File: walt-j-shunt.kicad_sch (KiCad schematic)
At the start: 32 parts, among them Q1 NMOS, Q2 NJVMJD45H11T4G, Q3 PNP, U1 AD817

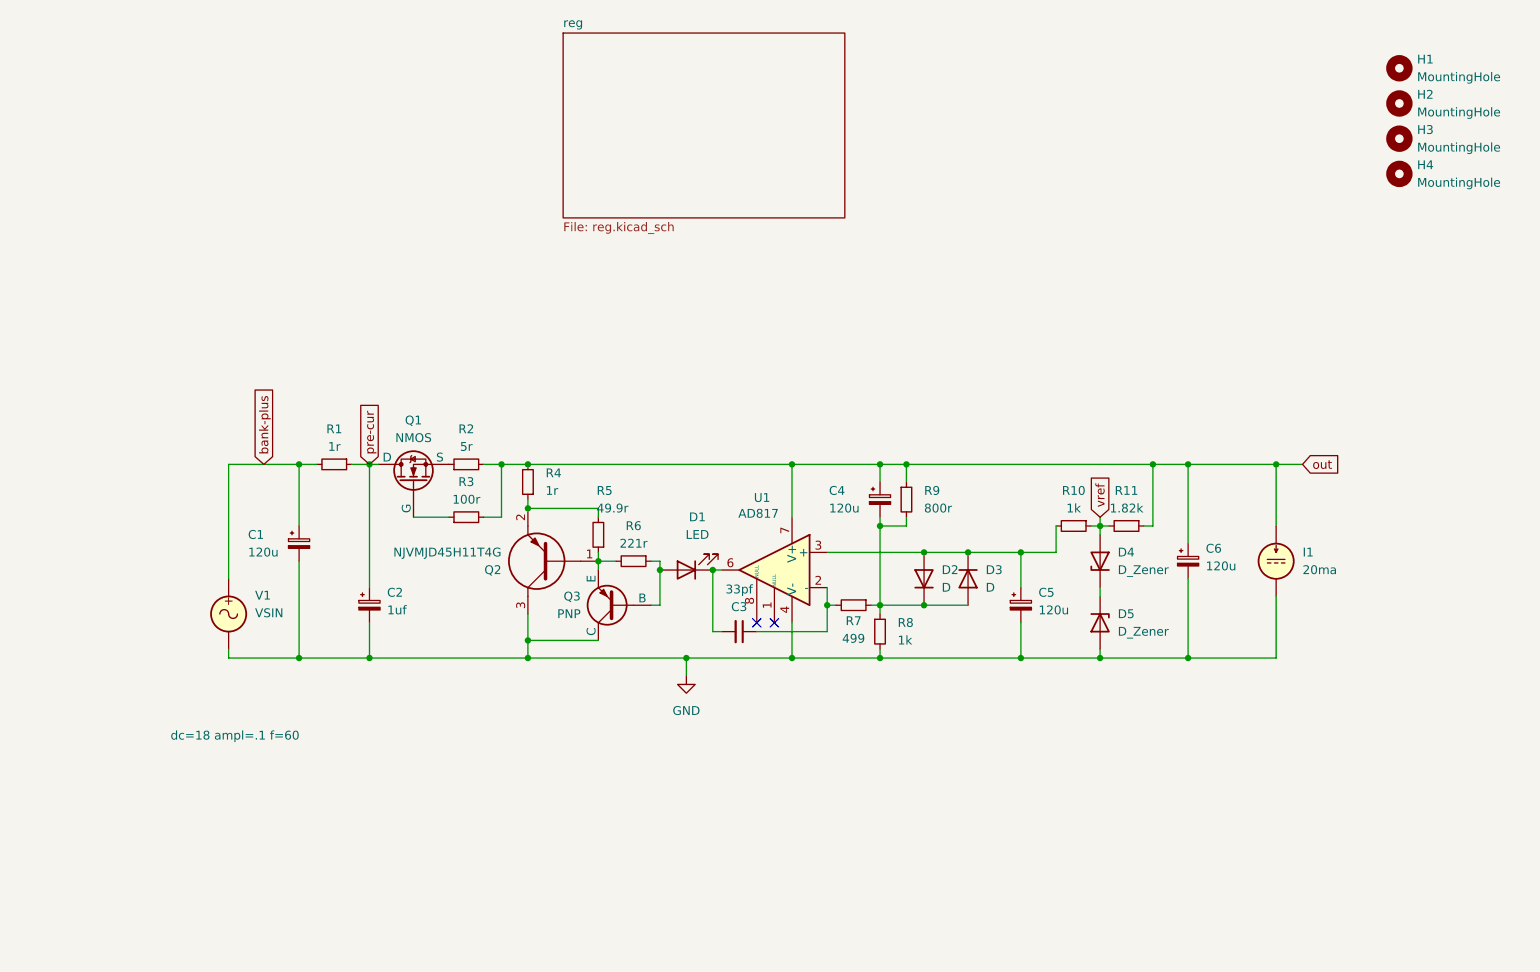
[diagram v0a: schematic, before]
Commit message: bipolar. untested
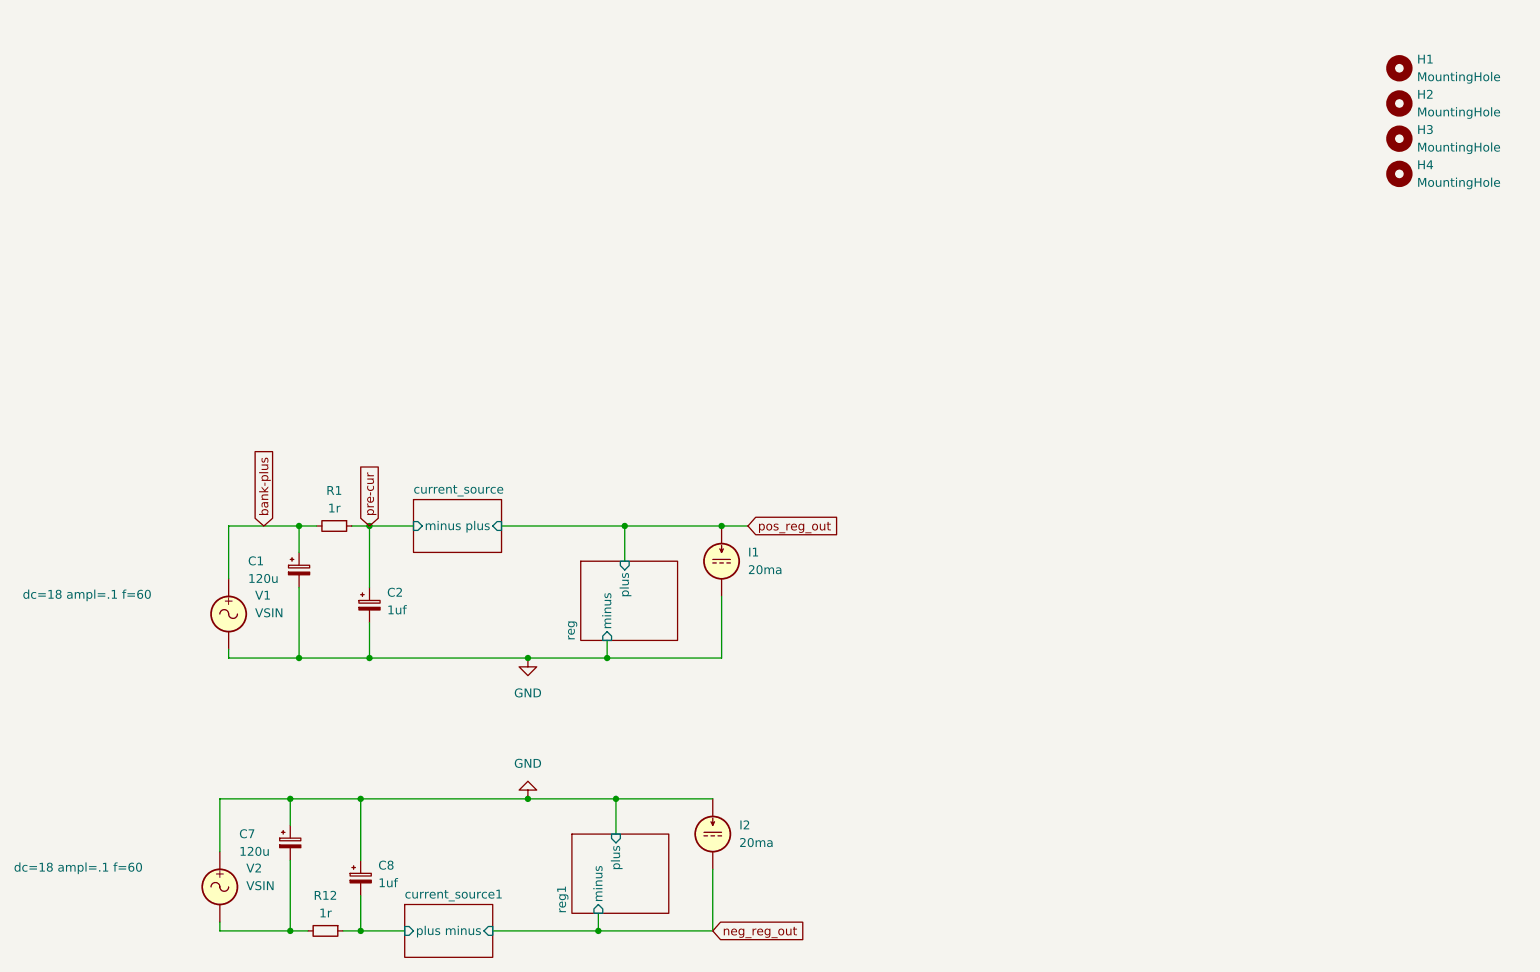
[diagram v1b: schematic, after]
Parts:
- removed C3: 33pf, Capacitor_SMD:C_0805_2012Metric, symbol Device:C_Small
- removed C4, C5, C6: 120u, Capacitor_THT:CP_Radial_D5.0mm_P2.00mm, symbol Device:C_Polarized_Small
- removed D1: LED, Diode_SMD:D_0805_2012Metric, symbol Device:LED
- removed D2, D3: D, Diode_SMD:D_SOD-123F, symbol Device:D
- removed D4, D5: D_Zener, Diode_SMD:D_MiniMELF, symbol Device:D_Zener
- removed Q1: NMOS, Package_TO_SOT_THT:TO-220-3_Horizontal_TabDown, symbol Simulation_SPICE:NMOS
- removed Q2: NJVMJD45H11T4G, Samacsys:DPAK_(SINGLE-GAUGE)_TO-252(369C)_ISSUE_F, symbol Samacsys:NJVMJD45H11T4G
- removed Q3: PNP, Package_TO_SOT_SMD:SOT-23-3, symbol Simulation_SPICE:PNP
- removed R10: 1k, Resistor_SMD:R_1206_3216Metric, symbol Device:R_Small
- removed R11: 1.82k, Resistor_SMD:R_1206_3216Metric, symbol Device:R_Small
- removed R2: 5r, Resistor_SMD:R_1206_3216Metric, symbol Device:R_Small
- removed R3: 100r, Resistor_SMD:R_1206_3216Metric, symbol Device:R_Small
- removed R4: 1r, Resistor_SMD:R_1206_3216Metric, symbol Device:R_Small
- removed R5: 49.9r, Resistor_SMD:R_1206_3216Metric, symbol Device:R_Small
- removed R6: 221r, Resistor_SMD:R_1206_3216Metric, symbol Device:R_Small
- removed R7: 499, Resistor_SMD:R_1206_3216Metric, symbol Device:R_Small
- removed R8: 1k, Resistor_SMD:R_MELF_MMB-0207, symbol Device:R_Small
- removed R9: 800r, Resistor_SMD:R_MELF_MMB-0207, symbol Device:R_Small
- removed U1: AD817, Package_SO:SOIC-8_3.9x4.9mm_P1.27mm, symbol Amplifier_Operational:AD817
- added C7: 120u, Capacitor_THT:CP_Radial_D5.0mm_P2.00mm, symbol Device:C_Polarized_Small
- added C8: 1uf, Samacsys:B32529C105J, symbol Device:C_Polarized_Small
- added I2: 20ma, Samacsys:395443002, symbol Simulation_SPICE:IDC
- added R12: 1r, Resistor_SMD:R_1206_3216Metric, symbol Device:R_Small
- added V2: VSIN, Samacsys:395443002, symbol Simulation_SPICE:VSIN
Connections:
- net GND: now also C7.1, C8.1, I2.1, V2.1
- net out renamed pos_reg_out
- new net: C7.2, R12.2, V2.2
- new net current_source1/plus: C8.2, R12.1
- new net neg_reg_out: I2.2
- no-connect marks 2 -> 0
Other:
- added sheet current_source (current_source.kicad_sch)
- added sheet current_source1 (current_source.kicad_sch)
- added sheet reg1 (reg.kicad_sch)
- sheet reg ports: added minus, plus; removed none
- moved on the sheet: C1, I1, R1
